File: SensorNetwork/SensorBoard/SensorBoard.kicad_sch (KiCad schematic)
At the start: 11 parts

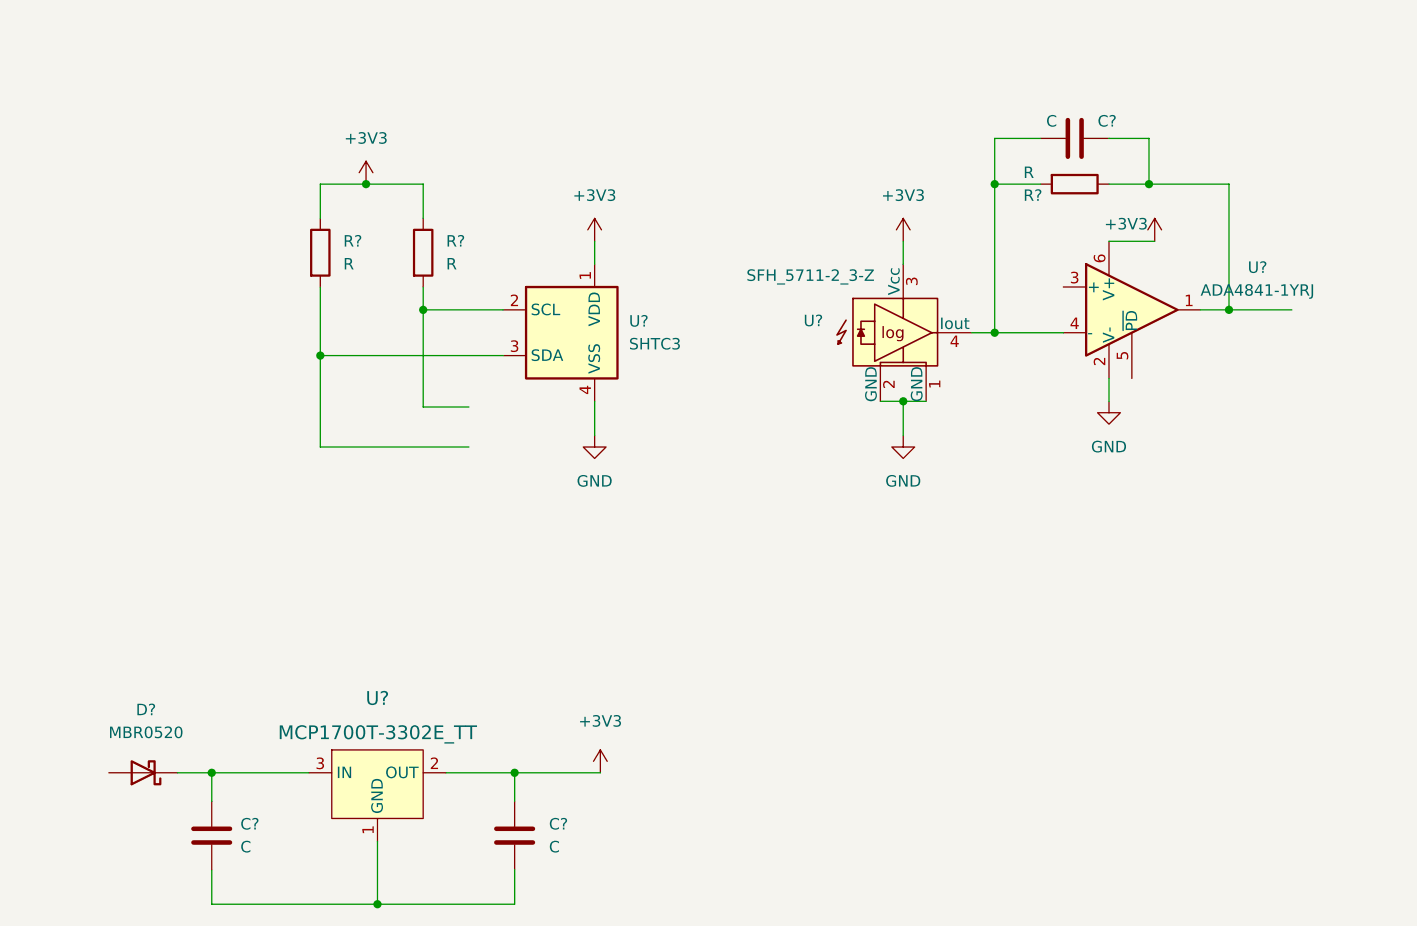
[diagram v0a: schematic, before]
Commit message: Sensor board routed and checked
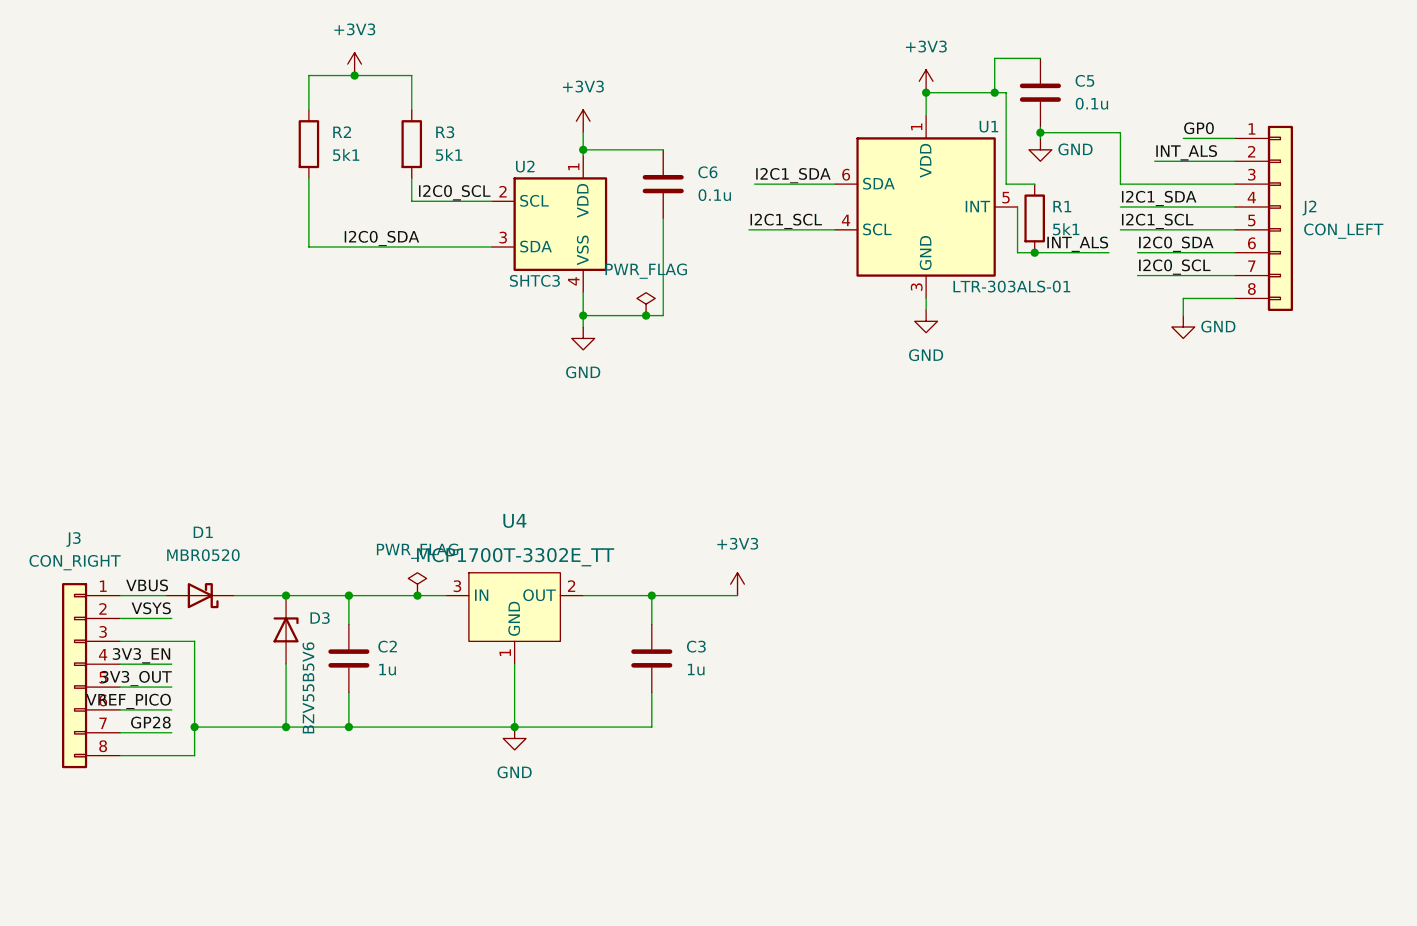
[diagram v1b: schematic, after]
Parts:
- removed C?: C, symbol Device:C
- removed R?: R, symbol Device:R
- removed U?: SFH_5711-2_3-Z, digikey-footprints:4-SMD_2.35x2.95mm, symbol dk_Optical-Sensors-Ambient-Light-IR-UV-Sensors:SFH_5711-2_3-Z
- removed U?: ADA4841-1YRJ, Package_TO_SOT_SMD:SOT-23-6, symbol Amplifier_Operational:ADA4841-1YRJ
- added C5, C6: 0.1u, Capacitor_SMD:C_0805_2012Metric, symbol Device:C
- added D3: BZV55B5V6, Diode_SMD:D_MiniMELF, symbol Diode:BZV55B5V6
- added J2: CON_LEFT, Connector_PinHeader_2.54mm:PinHeader_1x08_P2.54mm_Vertical, symbol Connector_Generic:Conn_01x08
- added J3: CON_RIGHT, Connector_PinHeader_2.54mm:PinHeader_1x08_P2.54mm_Vertical, symbol Connector_Generic:Conn_01x08
- added R1: 5k1, Resistor_SMD:R_0603_1608Metric, symbol Device:R
- added U1: LTR-303ALS-01, OptoDevice:Lite-On_LTR-303ALS-01, symbol Sensor_Optical:LTR-303ALS-01
- C2, C3: renamed from C?; value C -> 1u; footprint (none) -> Capacitor_SMD:C_0805_2012Metric
- R2, R3: renamed from R?; value R -> 5k1; footprint (none) -> Resistor_SMD:R_0603_1608Metric
- gave numbers to parts that had none: 3
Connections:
- net +3V3: now also C5.1, C6.1, R1.1, U1.1 (VDD)
- net GND: now also C2.2, C3.2, U4.1 (GND), C5.2, C6.2, D3.2 (A), J2.3 (Pin_3), J2.8 (Pin_8), J3.3 (Pin_3), J3.8 (Pin_8), U1.3 (GND)
- net I2C0_SCL: now reaches R3.2, U2.2 (SCL)
- net I2C0_SCL: now also J2.7 (Pin_7)
- net I2C0_SDA: now reaches R2.2, U2.3 (SDA)
- net I2C0_SDA: now also J2.6 (Pin_6)
- net at C2.1, D1.1 (K), U4.3 (IN): now also D3.1 (K)
- net VBUS: now reaches D1.2 (A)
- net VBUS: now also J3.1 (Pin_1)
- new net 3V3_EN: J3.4 (Pin_4)
- new net 3V3_OUT: J3.5 (Pin_5)
- new net GP0: J2.1 (Pin_1)
- new net GP28: J3.7 (Pin_7)
- new net I2C1_SCL: J2.5 (Pin_5), U1.4 (SCL)
- new net I2C1_SDA: J2.4 (Pin_4), U1.6 (SDA)
- new net INT_ALS: J2.2 (Pin_2), R1.2, U1.5 (INT)
- new net VREF_PICO: J3.6 (Pin_6)
- new net VSYS: J3.2 (Pin_2)
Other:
- moved on the sheet: C2, C3, D1, R2, R3, U2, U4

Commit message: Documentation and specifications
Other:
- company: (none) -> 125 Systems
- title: (none) -> T RH LUX Sensor Board
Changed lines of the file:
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@@
 (kicad_sch (version 20211123) (generator eeschema)
   (paper "A5")
+  (title_block
+    (title "T RH LUX Sensor Board")
+    (date "04-JAN-2023")
+    (rev "1")
+    (company "125 Systems")
+    (comment 1 "Author: Neeraj Adsul")
+  )
   (junction (at 60.325 85.09) (diameter 0) (color 0 0 0 0)
   )
